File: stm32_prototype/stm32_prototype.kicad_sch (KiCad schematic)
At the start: 1 part, among them U1 STM32F103C8Tx

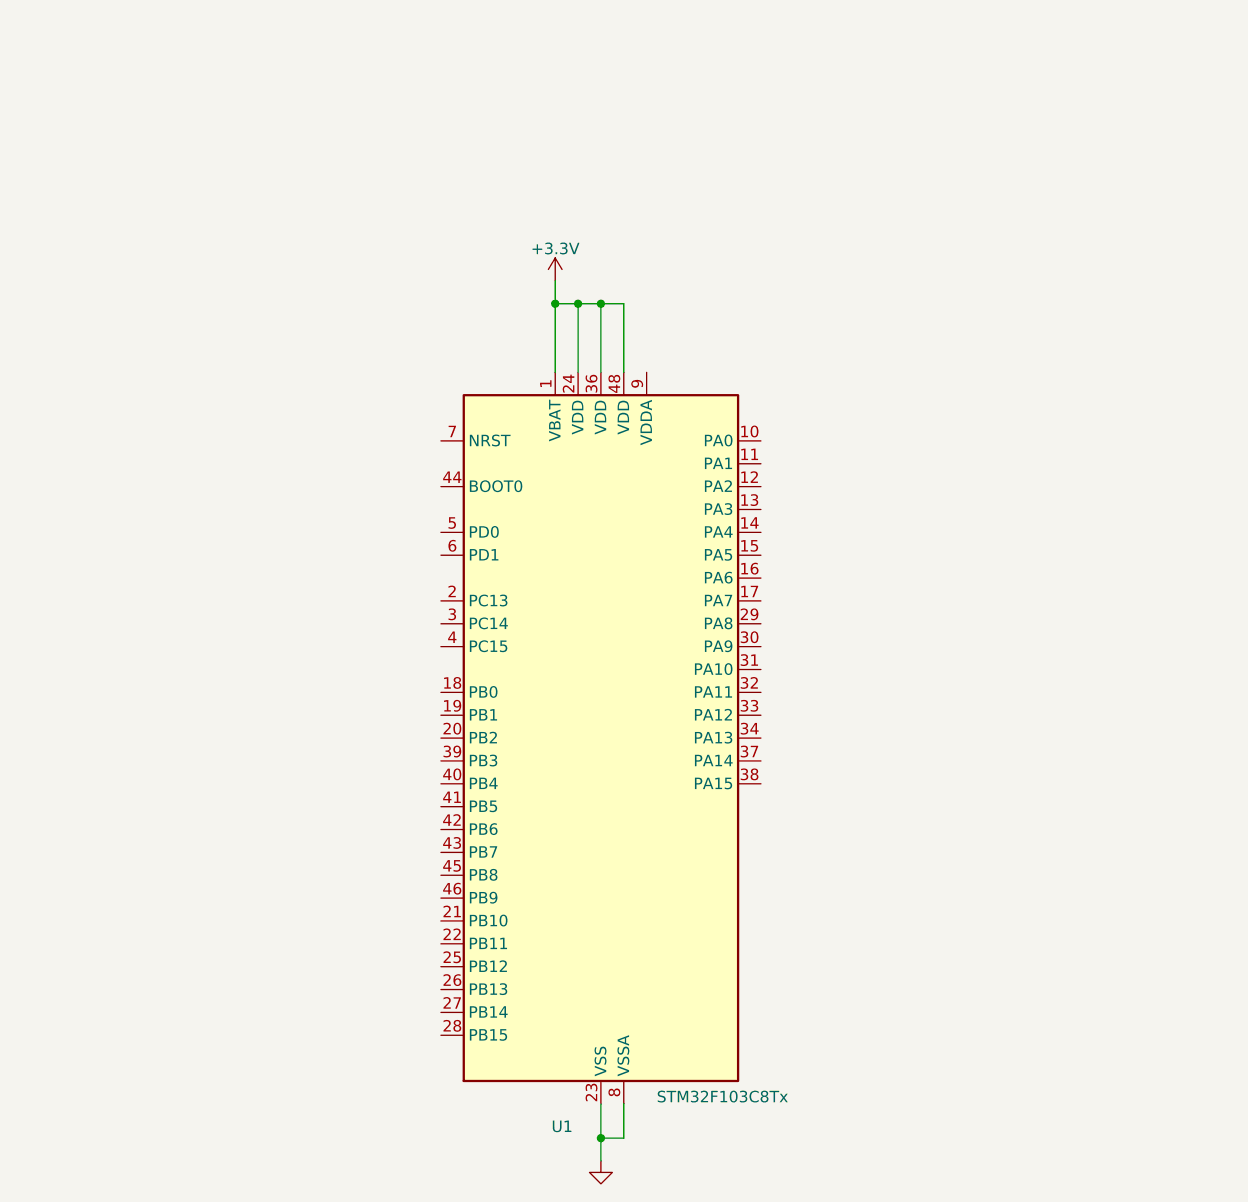
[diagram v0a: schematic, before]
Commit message: mkdocs..
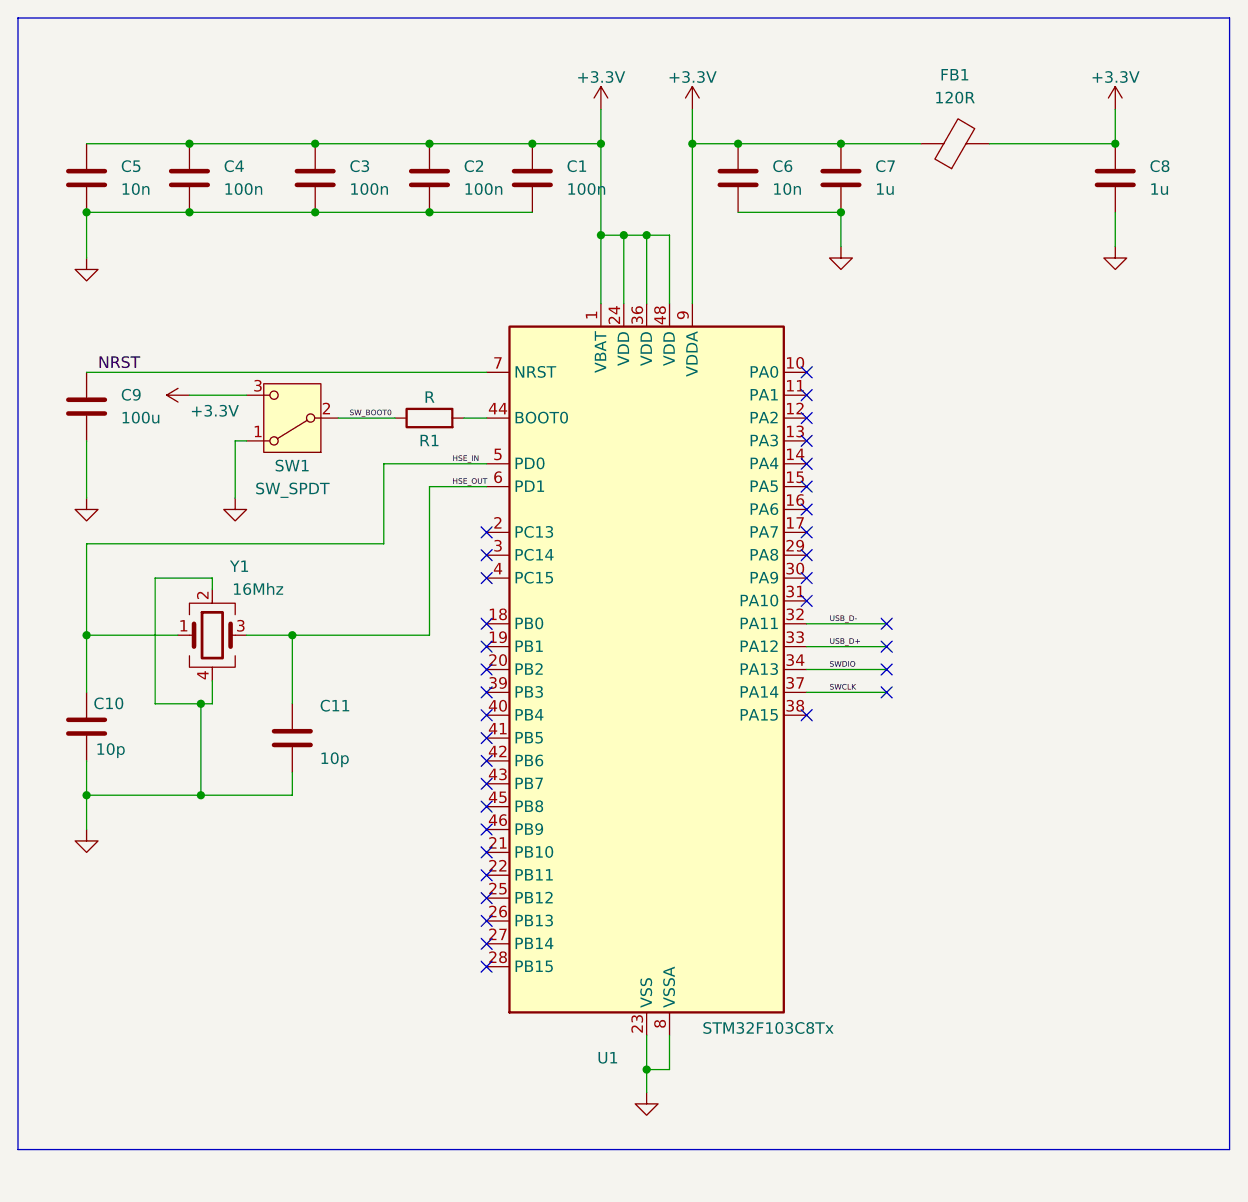
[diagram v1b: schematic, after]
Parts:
- added C1, C2, C3, C4: 100n, symbol Device:C
- added C10, C11: 10p, symbol Device:C
- added C5, C6: 10n, symbol Device:C
- added C7, C8: 1u, symbol Device:C
- added C9: 100u, symbol Device:C
- added FB1: 120R, symbol Device:FerriteBead
- added R1: R, symbol Device:R
- added SW1: SW_SPDT, symbol Switch:SW_SPDT
- added Y1: 16Mhz, symbol Device:Crystal_GND24
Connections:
- net +3.3V: now also U1.9 (VDDA), C1.1, C2.1, C3.1, C4.1, C5.1, C6.1, C7.1, C8.1, FB1.1, FB1.2, SW1.3 (C)
- net GND: now also C1.2, C10.2, C11.2, C2.2, C3.2, C4.2, C5.2, C6.2, C7.2, C8.2, C9.2, SW1.1 (A), Y1.2, Y1.4
- net USB_D-: now reaches U1.32 (PA11)
- net USB_D+: now reaches U1.33 (PA12)
- net SWDIO: now reaches U1.34 (PA13)
- net SWCLK: now reaches U1.37 (PA14)
- net at U1.44 (BOOT0): now also R1.2
- net HSE_IN: now reaches U1.5 (PD0)
- net HSE_IN: now also C10.1, Y1.1
- net HSE_OUT: now reaches U1.6 (PD1)
- net HSE_OUT: now also C11.1, Y1.3
- net NRST: now reaches U1.7 (NRST)
- net NRST: now also C9.1
- new net SW_BOOT0: R1.1, SW1.2 (B)
- no-connect marks 0 -> 35
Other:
- moved on the sheet: U1
